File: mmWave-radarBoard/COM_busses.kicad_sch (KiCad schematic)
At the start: 31 parts, among them J401 Conn_01x03_Socket, J402 Conn_01x03_Socket, J403 Conn_01x03_Socket, U401 TCAN1042HGVDRQ1, U402 TLIN1039DDFRQ1, U403 TRS3221EIDBR

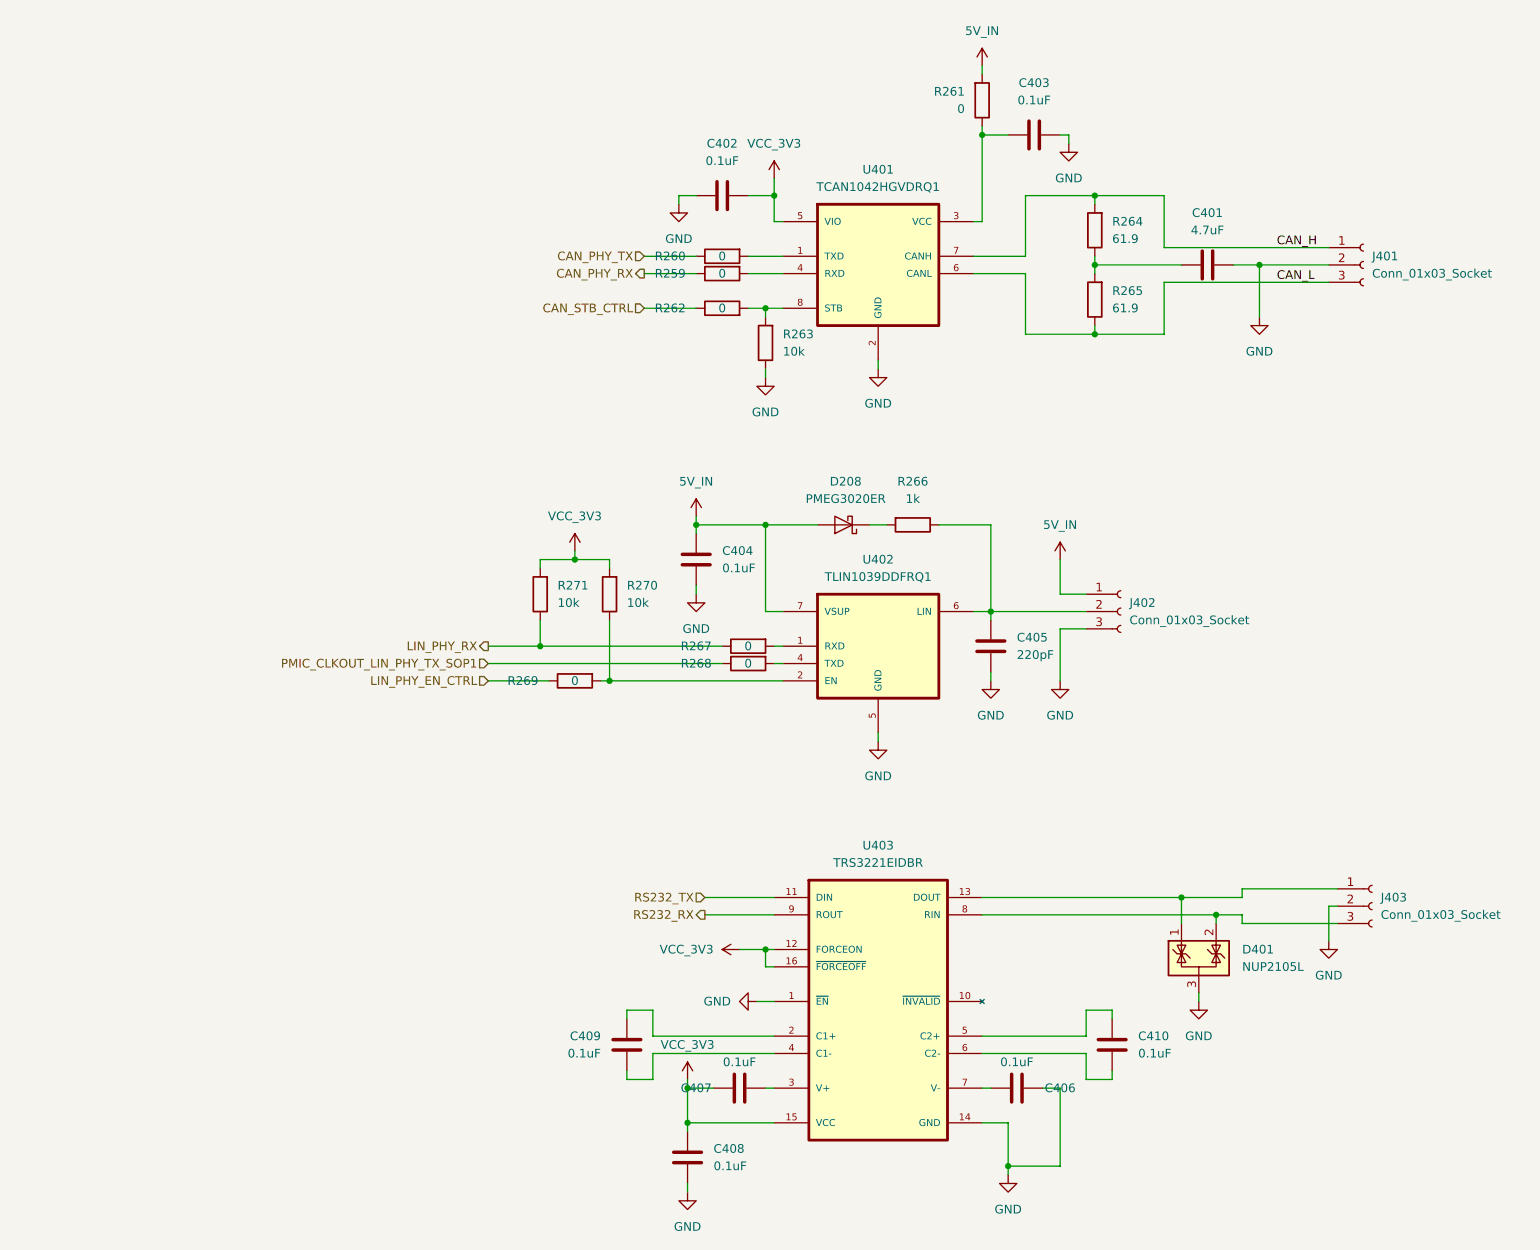
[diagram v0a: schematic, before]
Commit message: Updated schematic
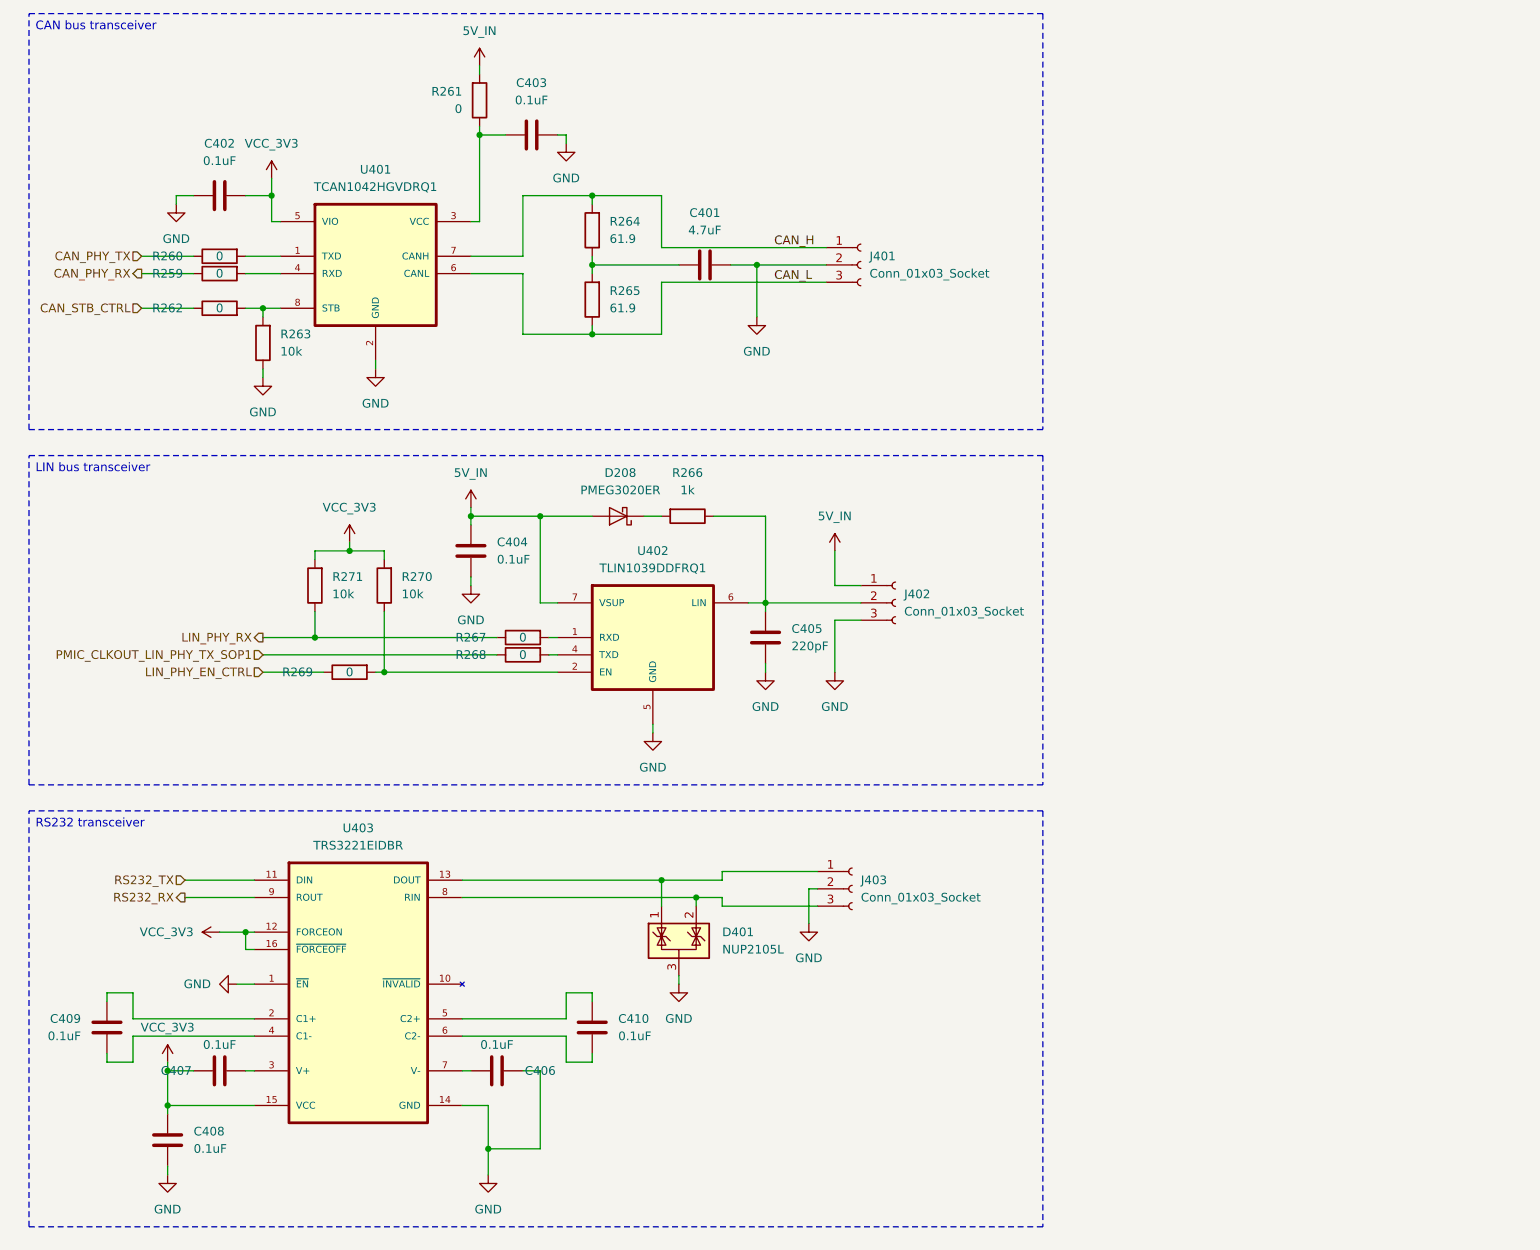
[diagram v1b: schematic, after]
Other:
- company: Emiel V -> Designer: EV
- moved on the sheet: C401, C402, C403, C404, C405, C406, C407, C408, C409, C410, D208, D401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
